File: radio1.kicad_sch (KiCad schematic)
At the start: 27 parts, among them U10 CC1125RHBR, Y3 OW2EL89CENUXK7YLC-40M

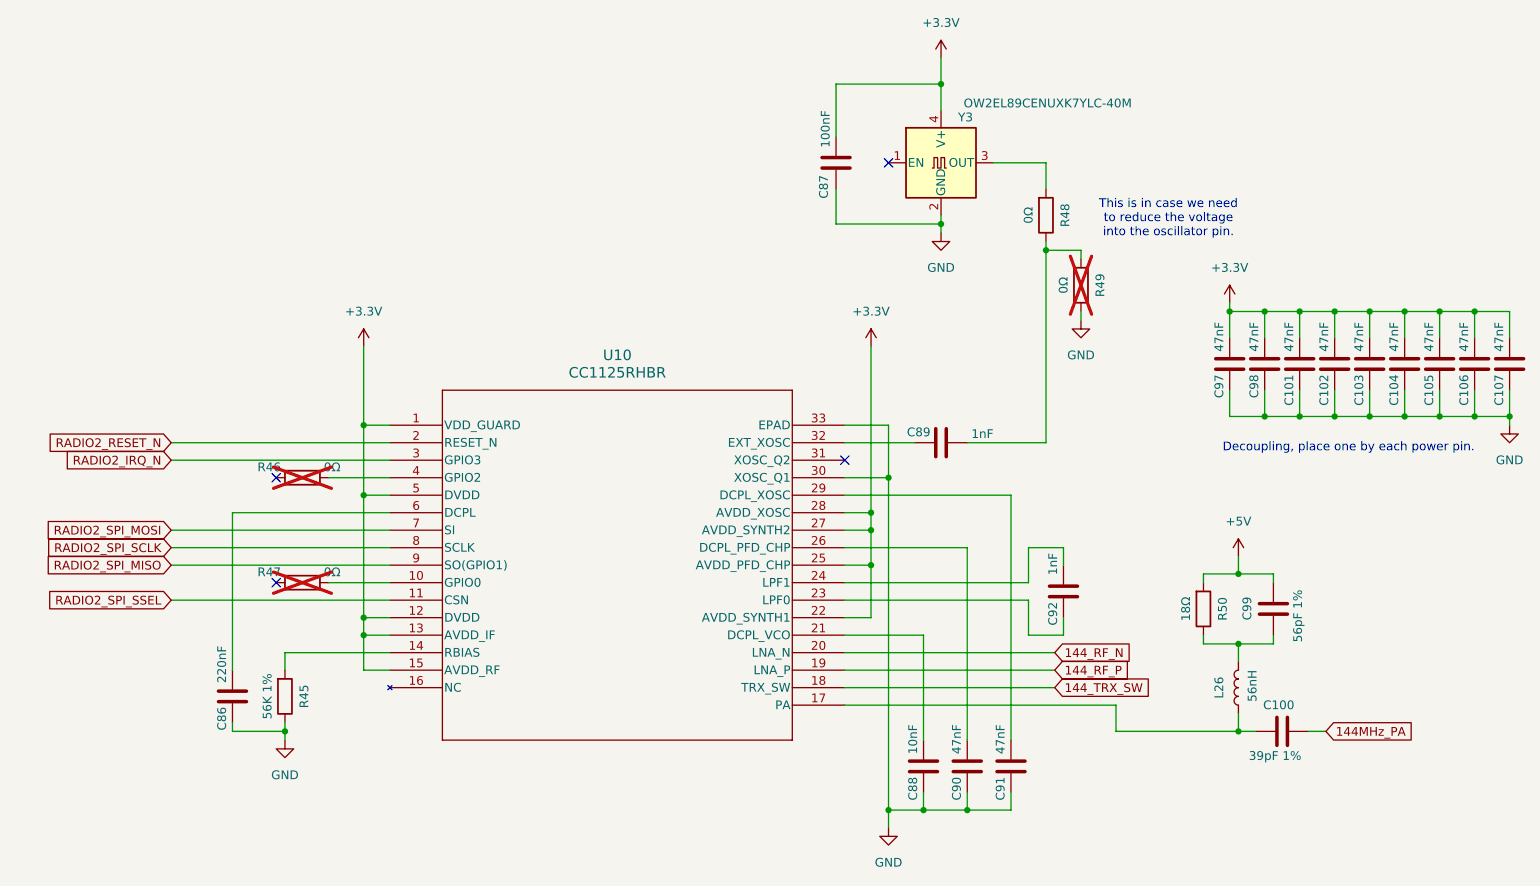
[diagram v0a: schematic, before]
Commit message: More re-layout for the new design
Signed-off-by: Corey Minyard <corey@minyard.net>
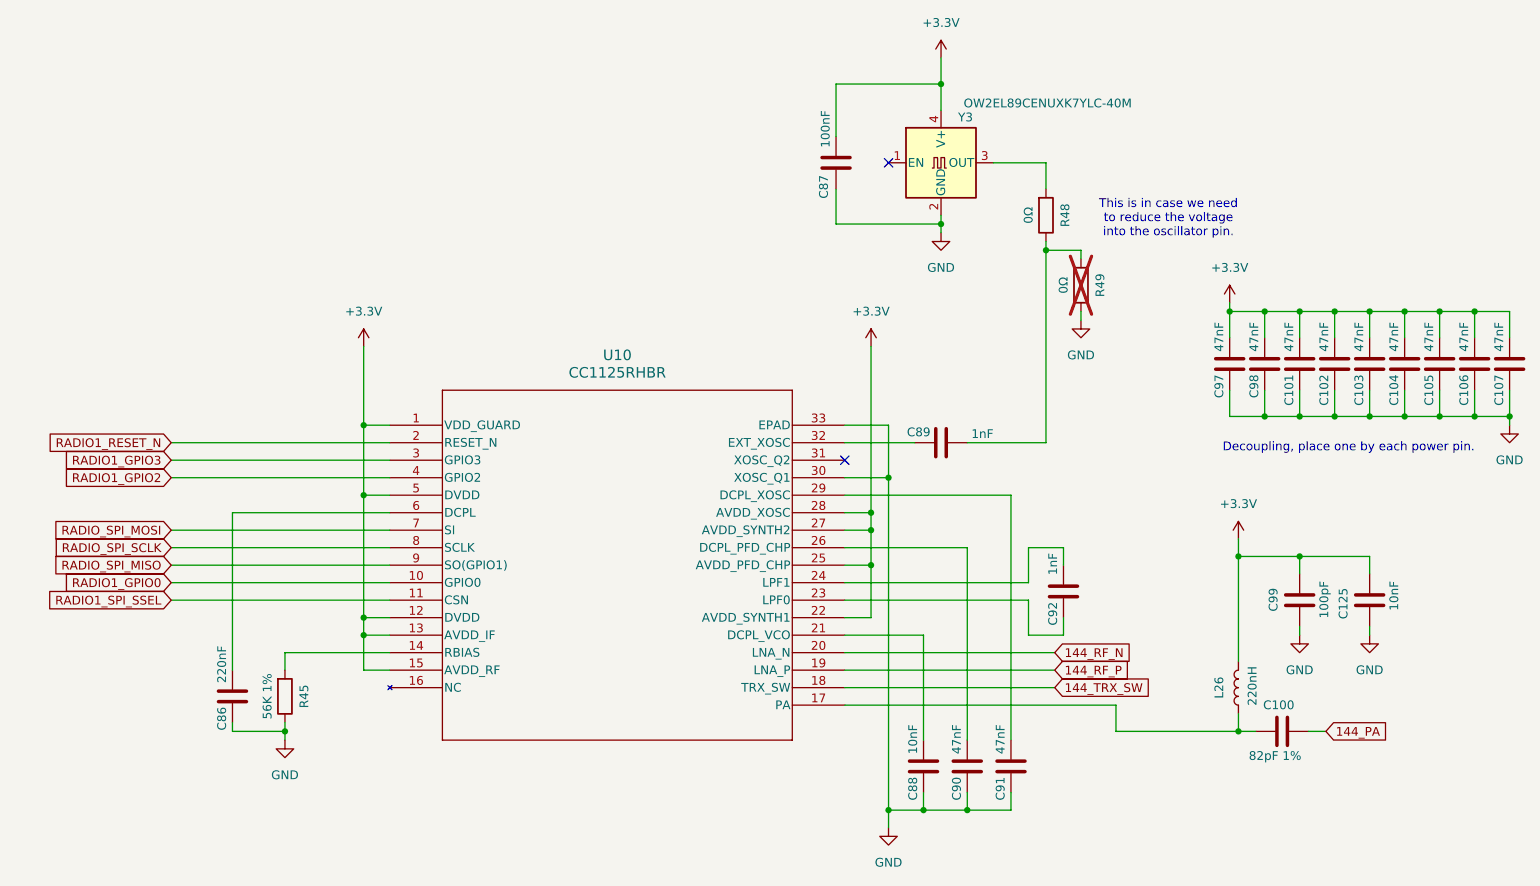
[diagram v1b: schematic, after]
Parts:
- removed R46, R47: 0Ω, Resistor_SMD:R_0402_1005Metric, symbol Device:R
- removed R50: 18Ω, Resistor_SMD:R_0402_1005Metric, symbol Device:R
- added C125: 10nF, Capacitor_SMD:C_0402_1005Metric_Pad0.74x0.62mm_HandSolder, symbol Device:C
- C100: value 39pF 1% -> 82pF 1%
- C99: value 56pF 1% -> 100pF
- L26: value 56nH -> 220nH
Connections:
- net +5V is gone; now on net +3.3V: C99.2
- net +3.3V: now also L26.2, C125.2
- net GND: now also C99.1, C125.1
- net RADIO1_GPIO2: now reaches U10.4 (GPIO2)
- net RADIO1_GPIO0: now reaches U10.10 (GPIO0)
- net 144MHz_PA renamed 144_PA
- net RADIO2_IRQ_N renamed RADIO1_GPIO3
- net RADIO2_RESET_N renamed RADIO1_RESET_N
- net RADIO2_SPI_MISO renamed RADIO_SPI_MISO
- net RADIO2_SPI_MOSI renamed RADIO_SPI_MOSI
- net RADIO2_SPI_SCLK renamed RADIO_SPI_SCLK
- net RADIO2_SPI_SSEL renamed RADIO1_SPI_SSEL
- no-connect marks 4 -> 2
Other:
- moved on the sheet: C99

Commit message: Add some vias
Signed-off-by: Corey Minyard <corey@minyard.net>
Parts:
- L26: footprint Inductor_SMD:L_0603_1608Metric_Pad1.05x0.95mm_HandSolder -> Inductor_SMD:L_0805_2012Metric_Pad1.05x1.20mm_HandSolder
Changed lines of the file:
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@@
 			)
 		)
-		(property "Footprint" "Inductor_SMD:L_0603_1608Metric_Pad1.05x0.95mm_HandSolder"
+		(property "Footprint" "Inductor_SMD:L_0805_2012Metric_Pad1.05x1.20mm_HandSolder"
 			(at 214.63 113.03 0)
 			(effects
